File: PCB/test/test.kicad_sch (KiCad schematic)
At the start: 53 parts, among them CN5 UFL, U1 STM32WBxx_QFN48, U2 USBLC6-2SC6, U3 LD3985M33R, X1 NX2016_32MHz, X2 NX2012_32K768Hz

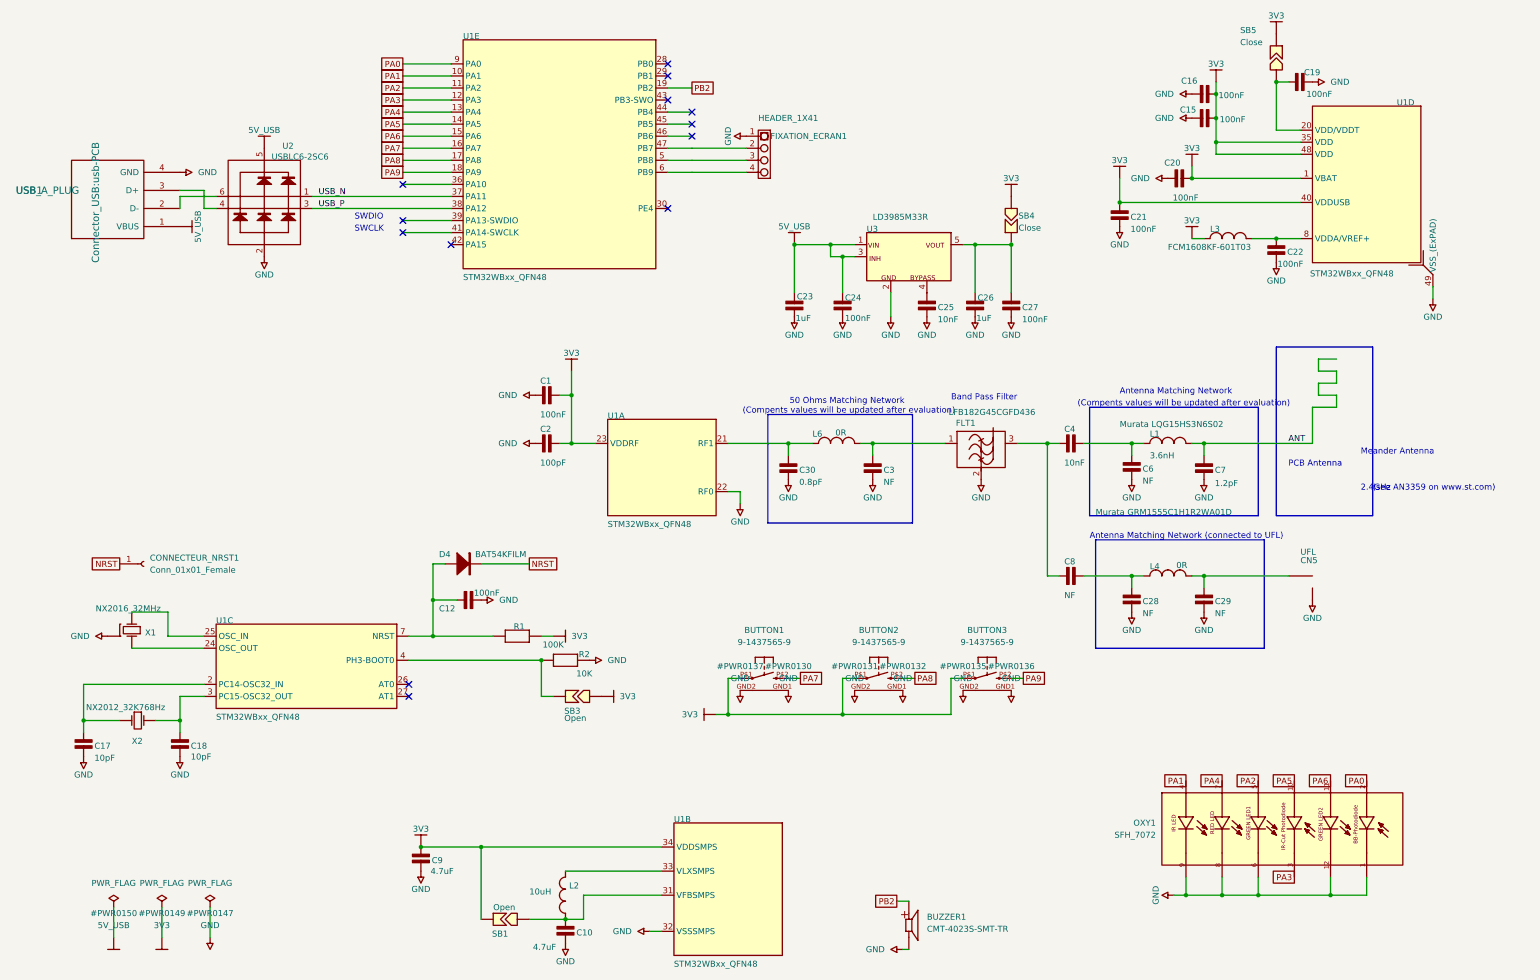
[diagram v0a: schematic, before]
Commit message: beaucoup de changements
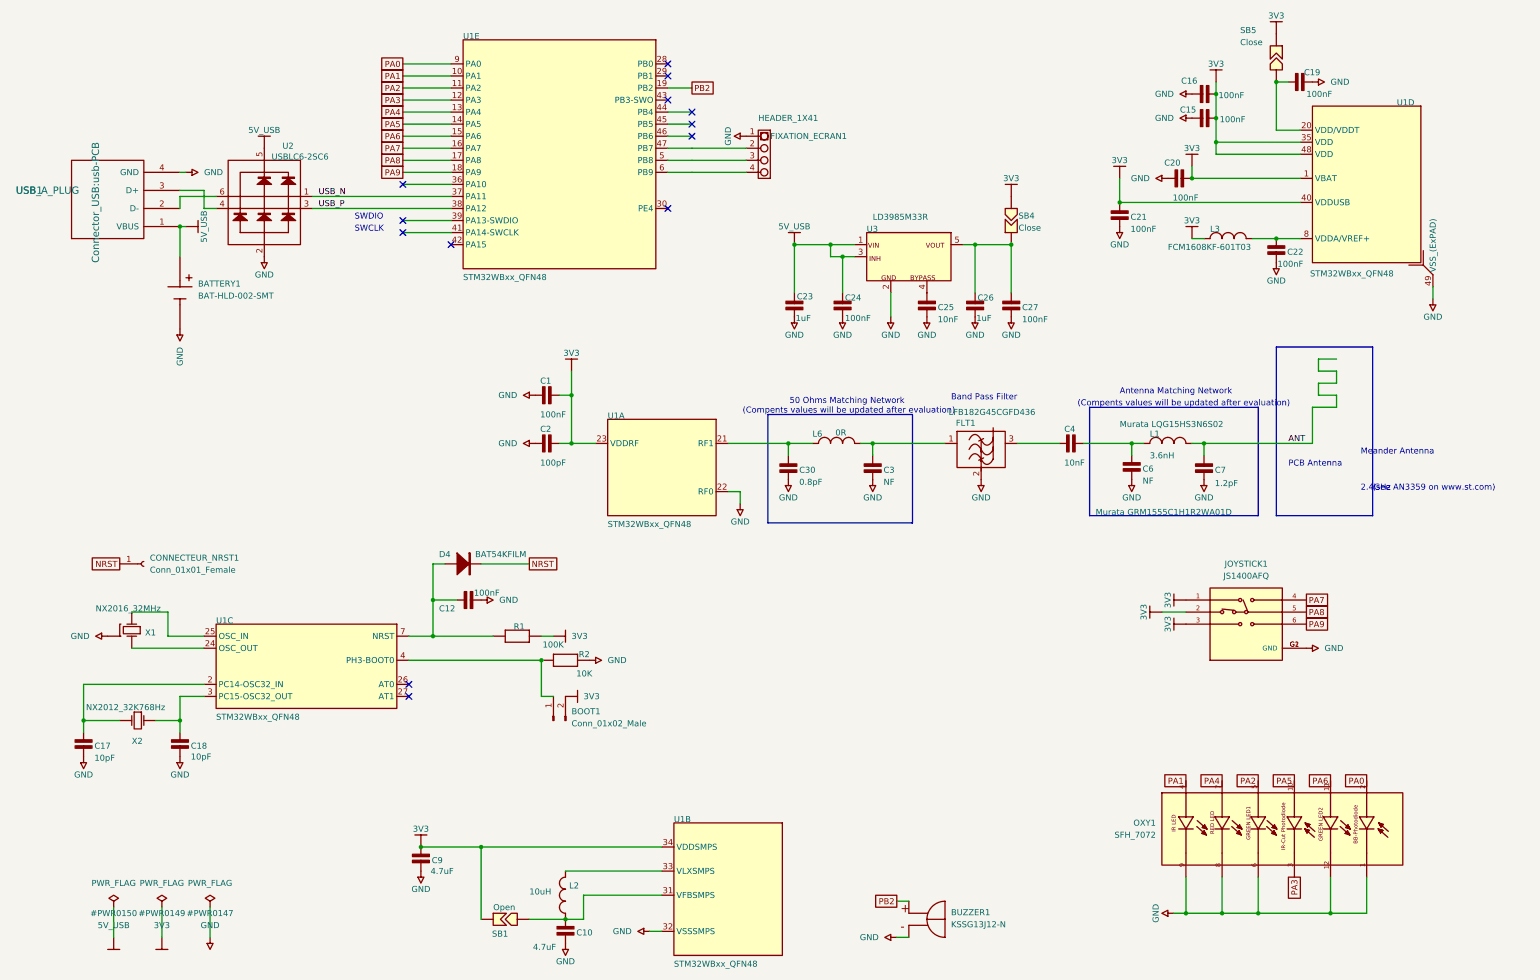
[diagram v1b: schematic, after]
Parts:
- removed BUTTON1, BUTTON2, BUTTON3: 9-1437565-9, FSMRACD, symbol 9-1437565-9:9-1437565-9
- removed BUZZER1: CMT-4023S-SMT-TR, CMT-4023S-SMT-TR:CUI_CMT-4023S-SMT-TR, symbol CMT-4023S-SMT-TR:CMT-4023S-SMT-TR
- removed C28, C29: NF, Library:0402_CAP_NPOL, symbol test-altium-import:0_CAP_NPOL
- removed C8: NF, Library:0402_CAP_NPOL, symbol test-altium-import:1_CAP_NPOL
- removed CN5: UFL, Library:UFL, symbol test-altium-import:0_mirrored_UFL
- removed L4: 0R, Library:0402_COIL, symbol test-altium-import:1_INDUCTOR_SMD_STDL
- removed SB3: Open, Library:SB-tiny, symbol test-altium-import:0_Strap2
- added BATTERY1: BAT-HLD-002-SMT, BAT_BAT-HLD-002-SMT, symbol BAT-HLD-002-SMT:BAT-HLD-002-SMT
- added BOOT1: Conn_01x02_Male, Connector_PinHeader_2.54mm:PinHeader_1x02_P2.54mm_Vertical, symbol Connector:Conn_01x02_Male
- added BUZZER1: KSSG13J12-N, XDCR_KSSG13J12-N, symbol KSSG13J12-N:KSSG13J12-N
- added JOYSTICK1: JS1400AFQ, SW_JS1400AFQ, symbol JS1400AFQ:JS1400AFQ
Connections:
- net 3V3: now also BOOT1.2 (Pin_2), JOYSTICK1.1, JOYSTICK1.2, JOYSTICK1.3
- net 5V_USB: now also BATTERY1.P1, BATTERY1.P2
- net GND: now also BATTERY1.N, BUZZER1.N, JOYSTICK1.G1 (GND), JOYSTICK1.G2 (GND)
- net PA7: now also JOYSTICK1.4
- net PA8: now also JOYSTICK1.5
- net PA9: now also JOYSTICK1.6
- net PB2: now also BUZZER1.P
- net at R2.1, U1.4 (PH3-BOOT0): now also BOOT1.1 (Pin_1)
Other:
- note removed: "Antenna Matching Network (connected to UFL)"
